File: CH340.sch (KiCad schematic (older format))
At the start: 10 parts, among them J5 USB_B_Micro, J7 Conn_01x04_Female_UART, U5 CH340C

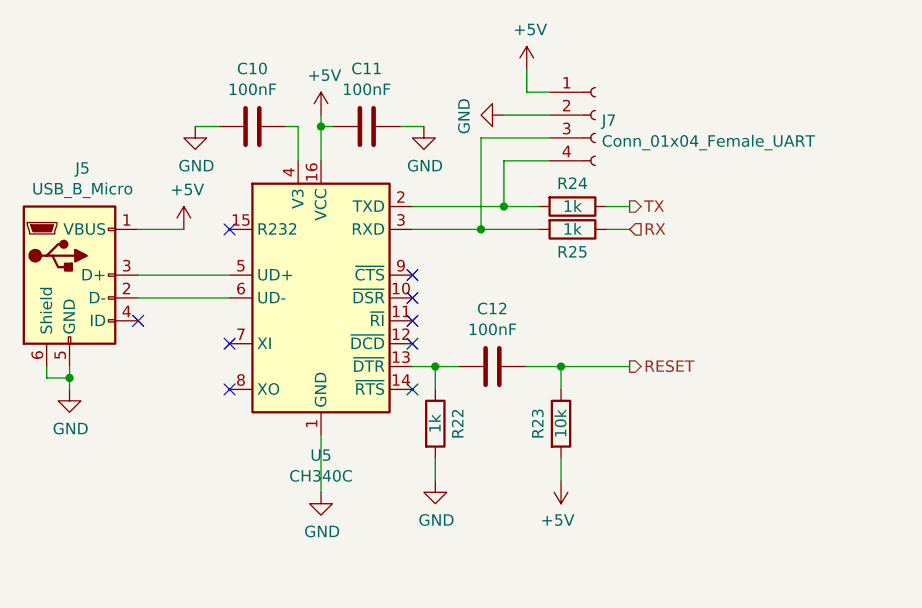
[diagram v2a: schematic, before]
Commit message: except GND
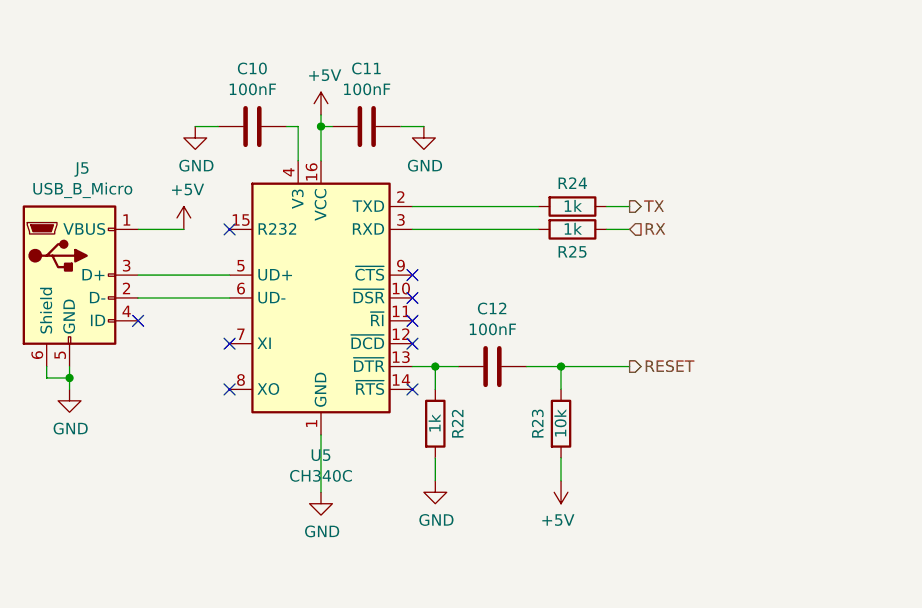
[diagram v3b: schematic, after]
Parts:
- removed J7: Conn_01x04_Female_UART, Connector_PinSocket_2.54mm:PinSocket_1x04_P2.54mm_Vertical, symbol Connector:Conn_01x04_Female
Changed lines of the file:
@@
 RESET
-Wire Wire Line
-	4550 1850 4950 1850
-Wire Wire Line
-	4550 1950 4850 1950
 Wire Wire Line
 	3350 2150 3750 2150
 Wire Wire Line
 	3350 2250 3750 2250
-$Comp
-L Connector:Conn_01x04_Female J7
-U 1 1 5E60C088
-P 5350 1450
-F 0 "J7" H 5378 1426 50  0000 L CNN
-F 1 "Conn_01x04_Female_UART" H 5378 1335 50  0000 L CNN
-F 2 "Connector_PinSocket_2.54mm:PinSocket_1x04_P2.54mm_Vertical" H 5350 1450 50  0001 C CNN
-F 3 "~" H 5350 1450 50  0001 C CNN
-	1    5350 1450
-	1    0    0    -1
-$EndComp
-Wire Wire Line
-	4950 1850 4950 1650
-Wire Wire Line
-	4950 1650 5150 1650
-Connection ~ 4950 1850
-Wire Wire Line
-	4950 1850 5100 1850
-Wire Wire Line
-	4850 1950 4850 1550
-Wire Wire Line
-	4850 1550 5150 1550
-Connection ~ 4850 1950
-Wire Wire Line
-	4850 1950 5100 1950
-$Comp
-L power:GND #PWR0171
-U 1 1 5E6138D2
-P 4950 1450
-F 0 "#PWR0171" H 4950 1200 50  0001 C CNN
-F 1 "GND" H 4955 1277 50  0000 C CNN
-F 2 "" H 4950 1450 50  0001 C CNN
-F 3 "" H 4950 1450 50  0001 C CNN
-	1    4950 1450
-	0    1    1    0
-$EndComp
-$Comp
-L power:+5V #PWR0172
-U 1 1 5E614188
-P 5050 1250
-F 0 "#PWR0172" H 5050 1100 50  0001 C CNN
-F 1 "+5V" H 5065 1423 50  0000 C CNN
-F 2 "" H 5050 1250 50  0001 C CNN
-F 3 "" H 5050 1250 50  0001 C CNN
-	1    5050 1250
-	1    0    0    -1
-$EndComp
-Wire Wire Line
-	4950 1450 5150 1450
-Wire Wire Line
-	5150 1350 5050 1350
-Wire Wire Line
-	5050 1350 5050 1250
 $Comp
 L power:+5V #PWR0173
@@
 Wire Wire Line
 	5200 2950 5200 3050
+Wire Wire Line
+	4550 1850 5100 1850
+Wire Wire Line
+	4550 1950 5100 1950
 $EndSCHEMATC

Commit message: v3.1
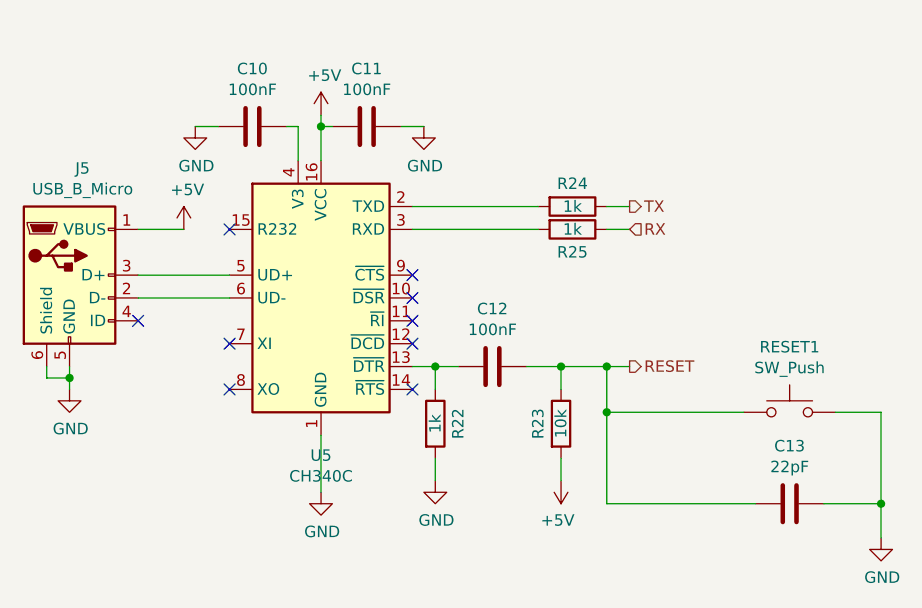
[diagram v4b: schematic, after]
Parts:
- added C13: 22pF, Capacitor_SMD:C_0603_1608Metric_Pad1.05x0.95mm_HandSolder, symbol Device:C
- added RESET1: SW_Push, Button_Switch_SMD:SW_SPST_TL3305A, symbol Switch:SW_Push
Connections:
- net GND: now also C13.1, RESET1.2
- net RESET: now also C13.2, RESET1.1
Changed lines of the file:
@@
 Connection ~ 5200 2550
 Wire Wire Line
-	5200 2550 5500 2550
+	5200 2550 5400 2550
 Wire Wire Line
 	5200 2950 5200 3050
@@
 Wire Wire Line
 	4550 1950 5100 1950
+$Comp
+L Switch:SW_Push RESET1
+U 1 1 5E935DDC
+P 6200 2750
+F 0 "RESET1" H 6200 3035 50  0000 C CNN
+F 1 "SW_Push" H 6200 2944 50  0000 C CNN
+F 2 "Button_Switch_SMD:SW_SPST_TL3305A" H 6200 2950 50  0001 C CNN
+F 3 "~" H 6200 2950 50  0001 C CNN
+	1    6200 2750
+	1    0    0    -1
+$EndComp
+$Comp
+L Device:C C13
+U 1 1 5E9386F1
+P 6200 3150
+F 0 "C13" V 5948 3150 50  0000 C CNN
+F 1 "22pF" V 6039 3150 50  0000 C CNN
+F 2 "Capacitor_SMD:C_0603_1608Metric_Pad1.05x0.95mm_HandSolder" H 6238 3000 50  0001 C CNN
+F 3 "~" H 6200 3150 50  0001 C CNN
+	1    6200 3150
+	0    1    1    0
+$EndComp
+$Comp
+L power:GND #PWR0167
+U 1 1 5E9394DF
+P 6600 3300
+F 0 "#PWR0167" H 6600 3050 50  0001 C CNN
+F 1 "GND" H 6605 3127 50  0000 C CNN
+F 2 "" H 6600 3300 50  0001 C CNN
+F 3 "" H 6600 3300 50  0001 C CNN
+	1    6600 3300
+	1    0    0    -1
+$EndComp
+Wire Wire Line
+	5400 2550 5400 2750
+Wire Wire Line
+	5400 3150 6050 3150
+Connection ~ 5400 2550
+Wire Wire Line
+	5400 2550 5500 2550
+Wire Wire Line
+	5400 2750 6000 2750
+Connection ~ 5400 2750
+Wire Wire Line
+	5400 2750 5400 3150
+Wire Wire Line
+	6400 2750 6600 2750
+Wire Wire Line
+	6600 2750 6600 3150
+Wire Wire Line
+	6350 3150 6600 3150
+Connection ~ 6600 3150
+Wire Wire Line
+	6600 3150 6600 3300
 $EndSCHEMATC
